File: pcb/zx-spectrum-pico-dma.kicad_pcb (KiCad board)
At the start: 2 copper layers, 99.9 x 98.2 mm, 2 parts, among them U101 RP2350_Stamp_XL

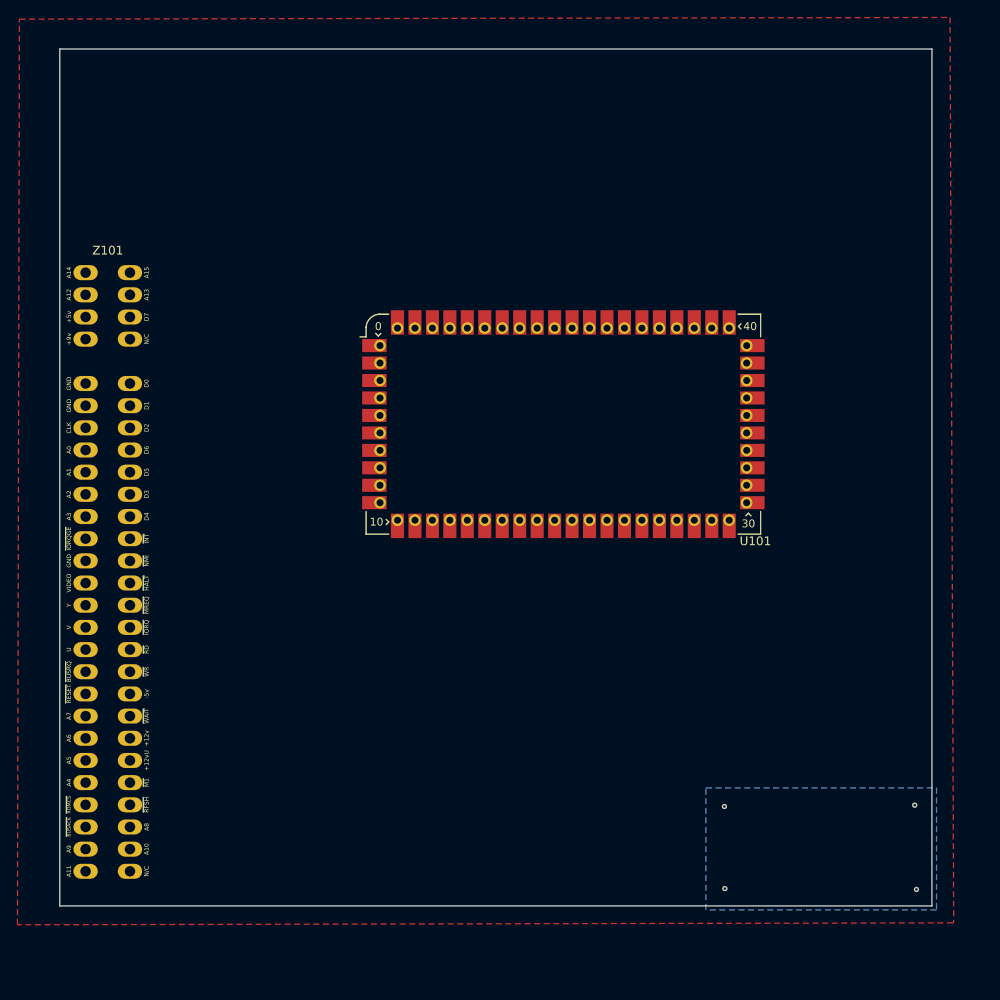
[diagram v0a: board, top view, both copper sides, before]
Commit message: more layout work
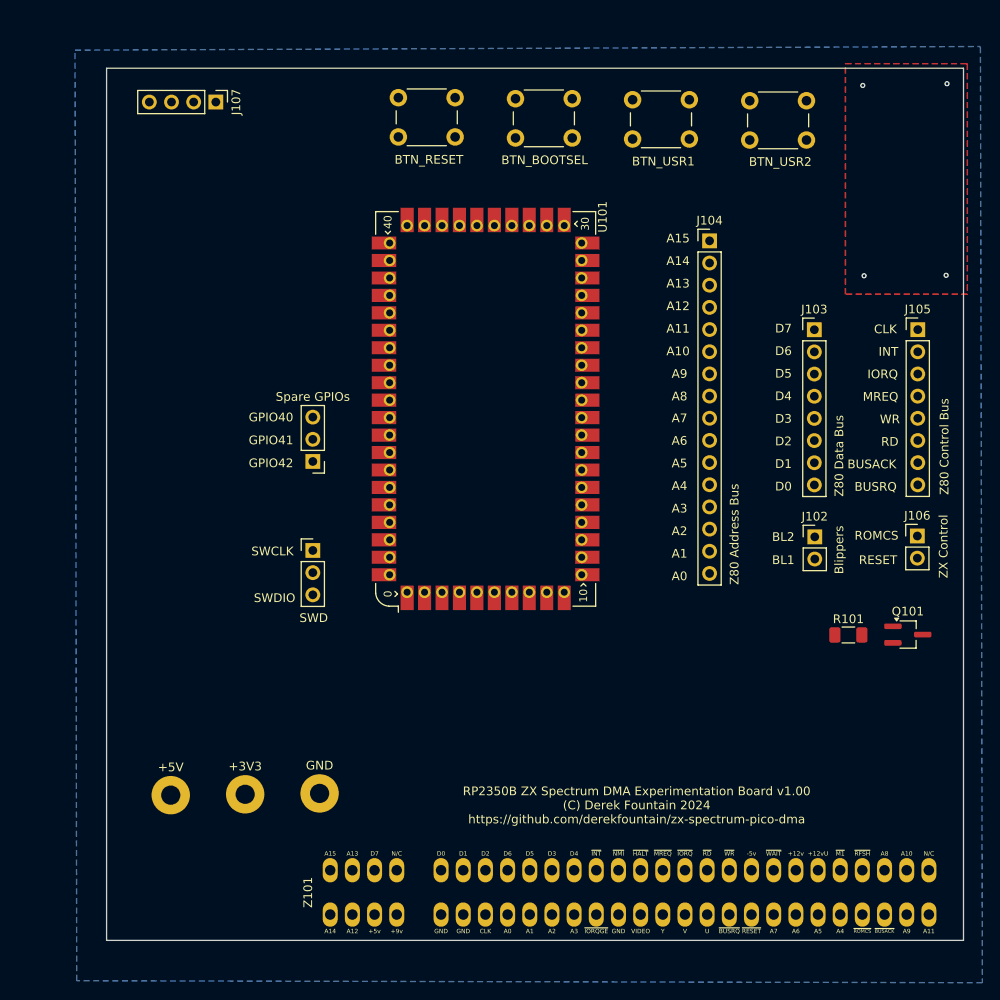
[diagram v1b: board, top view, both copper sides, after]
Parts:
- added H101: +5V, MountingHole:MountingHole_2.2mm_M2_Pad, F.Cu at (59.0, 136.3)
- added H102: +3V3, MountingHole:MountingHole_2.2mm_M2_Pad, F.Cu at (67.5, 136.2)
- added H103: GND, MountingHole:MountingHole_2.2mm_M2_Pad, F.Cu at (76.0, 136.2)
- added J101: SWD, Connector_PinHeader_2.54mm:PinHeader_1x03_P2.54mm_Vertical, F.Cu at (75.2, 108.3)
- added J102: Blippers, Connector_PinHeader_2.54mm:PinHeader_1x02_P2.54mm_Vertical, F.Cu at (132.8, 106.8)
- added J103: Z80 Data Bus, Connector_PinHeader_2.54mm:PinHeader_1x08_P2.54mm_Vertical, F.Cu at (132.7, 83.0)
- added J104: Z80 Address Bus, Connector_PinHeader_2.54mm:PinHeader_1x16_P2.54mm_Vertical, F.Cu at (120.7, 72.8)
- added J105: Z80 Control Bus, Connector_PinHeader_2.54mm:PinHeader_1x08_P2.54mm_Vertical, F.Cu at (144.6, 83.0)
- added J106: ZX Control, Connector_PinHeader_2.54mm:PinHeader_1x02_P2.54mm_Vertical, F.Cu at (144.5, 106.7)
- added J107: OLED, Connector_PinHeader_2.54mm:PinHeader_1x04_P2.54mm_Vertical, F.Cu at (64.1, 57.0)
- added J108: Spare GPIOs, Connector_PinHeader_2.54mm:PinHeader_1x03_P2.54mm_Vertical, F.Cu at (75.2, 98.1)
- added Q101: PMBT2222A, Package_TO_SOT_SMD:TSOT-23_HandSoldering, F.Cu at (143.4, 118.0)
- added R101: 1K, Resistor_SMD:R_1206_3216Metric_Pad1.30x1.75mm_HandSolder, F.Cu at (136.6, 118.0)
- added SW101: BTN_RESET, Button_Switch_THT:SW_PUSH_6mm_H4.3mm, F.Cu at (85.0, 56.5)
- added SW102: BTN_BOOTSEL, Button_Switch_THT:SW_PUSH_6mm_H4.3mm, F.Cu at (98.5, 56.6)
- added SW103: BTN_USR1, Button_Switch_THT:SW_PUSH_6mm_H4.3mm, F.Cu at (111.9, 56.7)
- added SW104: BTN_USR2, Button_Switch_THT:SW_PUSH_6mm_H4.3mm, F.Cu at (125.3, 56.8)
- moved Z101 69.7 mm to (110.3, 147.5), turned to 0 degrees
- moved U101 9.07 mm to (95.0, 92.1), turned to 90 degrees
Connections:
- U101 pad 1: unconnected-(U101A-GPIO0-Pad1) -> ZXD0
- U101 pad 10: unconnected-(U101A-GPIO9-Pad10) -> ZXA1
- U101 pad 11: unconnected-(U101A-GPIO10-Pad11) -> ZXA2
- U101 pad 12: unconnected-(U101A-GPIO11-Pad12) -> ZXA3
- U101 pad 13: unconnected-(U101A-GPIO12-Pad13) -> ZXA4
- U101 pad 14: unconnected-(U101A-GPIO13-Pad14) -> ZXA5
- U101 pad 15: unconnected-(U101A-GPIO14-Pad15) -> ZXA6
- U101 pad 16: unconnected-(U101A-GPIO15-Pad16) -> ZXA7
- U101 pad 17: unconnected-(U101A-GPIO16-Pad17) -> ZXA8
- U101 pad 18: unconnected-(U101A-GPIO17-Pad18) -> ZXA9
- U101 pad 19: unconnected-(U101A-GPIO18-Pad19) -> ZXA10
- U101 pad 2: unconnected-(U101A-GPIO1-Pad2) -> ZXD1
- U101 pad 20: unconnected-(U101A-GPIO19-Pad20) -> ZXA11
- U101 pad 21: unconnected-(U101A-GPIO20-Pad21) -> ZXA12
- U101 pad 22: unconnected-(U101A-GPIO21-Pad22) -> ZXA13
- U101 pad 23: unconnected-(U101A-GPIO22-Pad23) -> ZXA14
- U101 pad 24: unconnected-(U101A-GPIO23-Pad24) -> ZXA15
- U101 pad 25: unconnected-(U101A-GPIO24-Pad25) -> ZXCLK
- U101 pad 26: unconnected-(U101A-GPIO25-Pad26) -> ZXINT
- U101 pad 27: unconnected-(U101A-GPIO26-Pad27) -> ZXM1
- U101 pad 28: unconnected-(U101A-GPIO27-Pad28) -> ZXRD
- U101 pad 29: unconnected-(U101A-GPIO28-Pad29) -> ZXWR
- U101 pad 3: unconnected-(U101A-GPIO2-Pad3) -> ZXD2
- U101 pad 30: unconnected-(U101A-GPIO29-Pad30) -> ZXROMCS
- U101 pad 31: unconnected-(U101A-GND-Pad31) -> GND
- U101 pad 33: unconnected-(U101A-5V-Pad33) -> +5V
- U101 pad 34: unconnected-(U101A-3.3V-Pad34) -> +3V3
- U101 pad 37: unconnected-(U101A-SWDIO-Pad37) -> /SWDIO
- U101 pad 38: unconnected-(U101A-SWCLK-Pad38) -> /SWCLK
- U101 pad 39: unconnected-(U101A-~{RESET}-Pad39) -> /~{RESET}
- U101 pad 4: unconnected-(U101A-GPIO3-Pad4) -> ZXD3
- U101 pad 40: unconnected-(U101A-BOOTSEL-Pad40) -> /BOOTSEL
- U101 pad 41: unconnected-(U101B-GPIO30-Pad41) -> ZXMREQ
- U101 pad 42: unconnected-(U101B-GPIO31-Pad42) -> ZXIORQ
- U101 pad 43: unconnected-(U101B-GPIO32-Pad43) -> ZXBUSRQ
- U101 pad 44: unconnected-(U101B-GPIO33-Pad44) -> ZXBUSACK
- U101 pad 45: unconnected-(U101B-GPIO34-Pad45) -> ZXNMI
- U101 pad 46: unconnected-(U101B-GPIO35-Pad46) -> ZXHALT
- U101 pad 47: unconnected-(U101B-GPIO36-Pad47) -> ZXWAIT
- U101 pad 48: unconnected-(U101B-GPIO37-Pad48) -> ZXRESET
- U101 pad 49: unconnected-(U101B-GPIO38-Pad49) -> /I2C1_SDA
- U101 pad 5: unconnected-(U101A-GPIO4-Pad5) -> ZXD4
- U101 pad 50: unconnected-(U101B-GPIO39-Pad50) -> /I2C1_SCL
- U101 pad 51: unconnected-(U101B-GPIO40-Pad51) -> /GPIO40
- U101 pad 52: unconnected-(U101B-GPIO41-Pad52) -> /GPIO41
- U101 pad 53: unconnected-(U101B-GPIO42-Pad53) -> /GPIO42
- U101 pad 54: unconnected-(U101B-GPIO43-Pad54) -> /RESET_Z80
- U101 pad 55: unconnected-(U101B-GPIO44-Pad55) -> /BTN_USR1
- U101 pad 56: unconnected-(U101B-GPIO45-Pad56) -> /BTN_USR2
- U101 pad 57: unconnected-(U101B-GPIO46-Pad57) -> /BLIPPER1
- U101 pad 58: unconnected-(U101B-GPIO47-Pad58) -> /BLIPPER2
- U101 pad 6: unconnected-(U101A-GPIO5-Pad6) -> ZXD5
- U101 pad 7: unconnected-(U101A-GPIO6-Pad7) -> ZXD6
- U101 pad 8: unconnected-(U101A-GPIO7-Pad8) -> ZXD7
- U101 pad 9: unconnected-(U101A-GPIO8-Pad9) -> ZXA0
- Z101 pad A1: unconnected-(Z101-A15-PadA1) -> ZXA15
- Z101 pad A10: unconnected-(Z101-D5-PadA10) -> ZXD5
- Z101 pad A11: unconnected-(Z101-D3-PadA11) -> ZXD3
- Z101 pad A12: unconnected-(Z101-D4-PadA12) -> ZXD4
- Z101 pad A13: unconnected-(Z101-~{INT}-PadA13) -> ZXINT
- Z101 pad A14: unconnected-(Z101-~{NMI}-PadA14) -> ZXNMI
- Z101 pad A15: unconnected-(Z101-~{HALT}-PadA15) -> ZXHALT
- Z101 pad A16: unconnected-(Z101-~{MREQ}-PadA16) -> ZXMREQ
- Z101 pad A17: unconnected-(Z101-~{IORQ}-PadA17) -> ZXIORQ
- Z101 pad A18: unconnected-(Z101-~{RD}-PadA18) -> ZXRD
- Z101 pad A19: unconnected-(Z101-~{WR}-PadA19) -> ZXWR
- Z101 pad A2: unconnected-(Z101-A13-PadA2) -> ZXA13
- Z101 pad A21: unconnected-(Z101-~{WAIT}-PadA21) -> ZXWAIT
- Z101 pad A24: unconnected-(Z101-~{M1}-PadA24) -> ZXM1
- Z101 pad A26: unconnected-(Z101-A8-PadA26) -> ZXA8
- Z101 pad A27: unconnected-(Z101-A10-PadA27) -> ZXA10
- Z101 pad A3: unconnected-(Z101-D7-PadA3) -> ZXD7
- Z101 pad A6: unconnected-(Z101-D0-PadA6) -> ZXD0
- Z101 pad A7: unconnected-(Z101-D1-PadA7) -> ZXD1
- Z101 pad A8: unconnected-(Z101-D2-PadA8) -> ZXD2
- Z101 pad A9: unconnected-(Z101-D6-PadA9) -> ZXD6
- Z101 pad B1: unconnected-(Z101-A14-PadB1) -> ZXA14
- Z101 pad B10: unconnected-(Z101-A1-PadB10) -> ZXA1
- Z101 pad B11: unconnected-(Z101-A2-PadB11) -> ZXA2
- Z101 pad B12: unconnected-(Z101-A3-PadB12) -> ZXA3
- Z101 pad B14: unconnected-(Z101-GND-PadB14) -> GND
- Z101 pad B19: unconnected-(Z101-~{BUSRQ}-PadB19) -> ZXBUSRQ
- Z101 pad B2: unconnected-(Z101-A12-PadB2) -> ZXA12
- Z101 pad B20: unconnected-(Z101-~{RESET}-PadB20) -> ZXRESET
- Z101 pad B21: unconnected-(Z101-A7-PadB21) -> ZXA7
- Z101 pad B22: unconnected-(Z101-A6-PadB22) -> ZXA6
- Z101 pad B23: unconnected-(Z101-A5-PadB23) -> ZXA5
- Z101 pad B24: unconnected-(Z101-A4-PadB24) -> ZXA4
- Z101 pad B25: unconnected-(Z101-~{ROMCS}-PadB25) -> ZXROMCS
- Z101 pad B26: unconnected-(Z101-~{BUSACK}-PadB26) -> ZXBUSACK
- Z101 pad B27: unconnected-(Z101-A9-PadB27) -> ZXA9
- Z101 pad B28: unconnected-(Z101-A11-PadB28) -> ZXA11
- Z101 pad B3: unconnected-(Z101-+5v-PadB3) -> +5V
- Z101 pad B6: unconnected-(Z101-GND-PadB6) -> GND
- Z101 pad B7: unconnected-(Z101-GND-PadB7) -> GND
- Z101 pad B8: unconnected-(Z101-CLK-PadB8) -> ZXCLK
- Z101 pad B9: unconnected-(Z101-A0-PadB9) -> ZXA0
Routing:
- net GND: vias 0 -> 4
- net (no net): vias 4 -> 0
- added copper zone on B.Cu, net GND
- added copper zone on F.Cu, net GND
- removed copper zone on B.Cu, net (none)
- removed copper zone on F.Cu, net (none)
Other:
- board size 99.9 x 98.2 mm -> 98.2 x 99.9 mm
- board text added: "A0"
- board text added: "A1"
- board text added: "A10"
- board text added: "A11"
- board text added: "A12"
- board text added: "A13"
- board text added: "A14"
- board text added: "A15"
- board text added: "A2"
- board text added: "A3"
- board text added: "A4"
- board text added: "A5"
- board text added: "A6"
- board text added: "A7"
- board text added: "A8"
- board text added: "A9"
- board text added: "BL1"
- board text added: "BL2"
- board text added: "BUSACK"
- board text added: "BUSRQ"
- board text added: "CLK"
- board text added: "D0"
- board text added: "D1"
- board text added: "D2"
- board text added: "D3"
- board text added: "D4"
- board text added: "D5"
- board text added: "D6"
- board text added: "D7"
- board text added: "GPIO40"
- board text added: "GPIO41"
- board text added: "GPIO42"
- board text added: "INT"
- board text added: "IORQ"
- board text added: "MREQ"
- board text added: "RD"
- board text added: "RESET"
- board text added: "ROMCS"
- board text added: "RP2350B ZX Spectrum DMA Experimentation Board v1.00 (C) Derek Fountain 2024 https://github.com/derekfountain/zx-spectrum-pico-dma"
- board text added: "SWCLK"
- board text added: "SWDIO"
- board text added: "WR"
